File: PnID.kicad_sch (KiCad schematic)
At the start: 14 parts

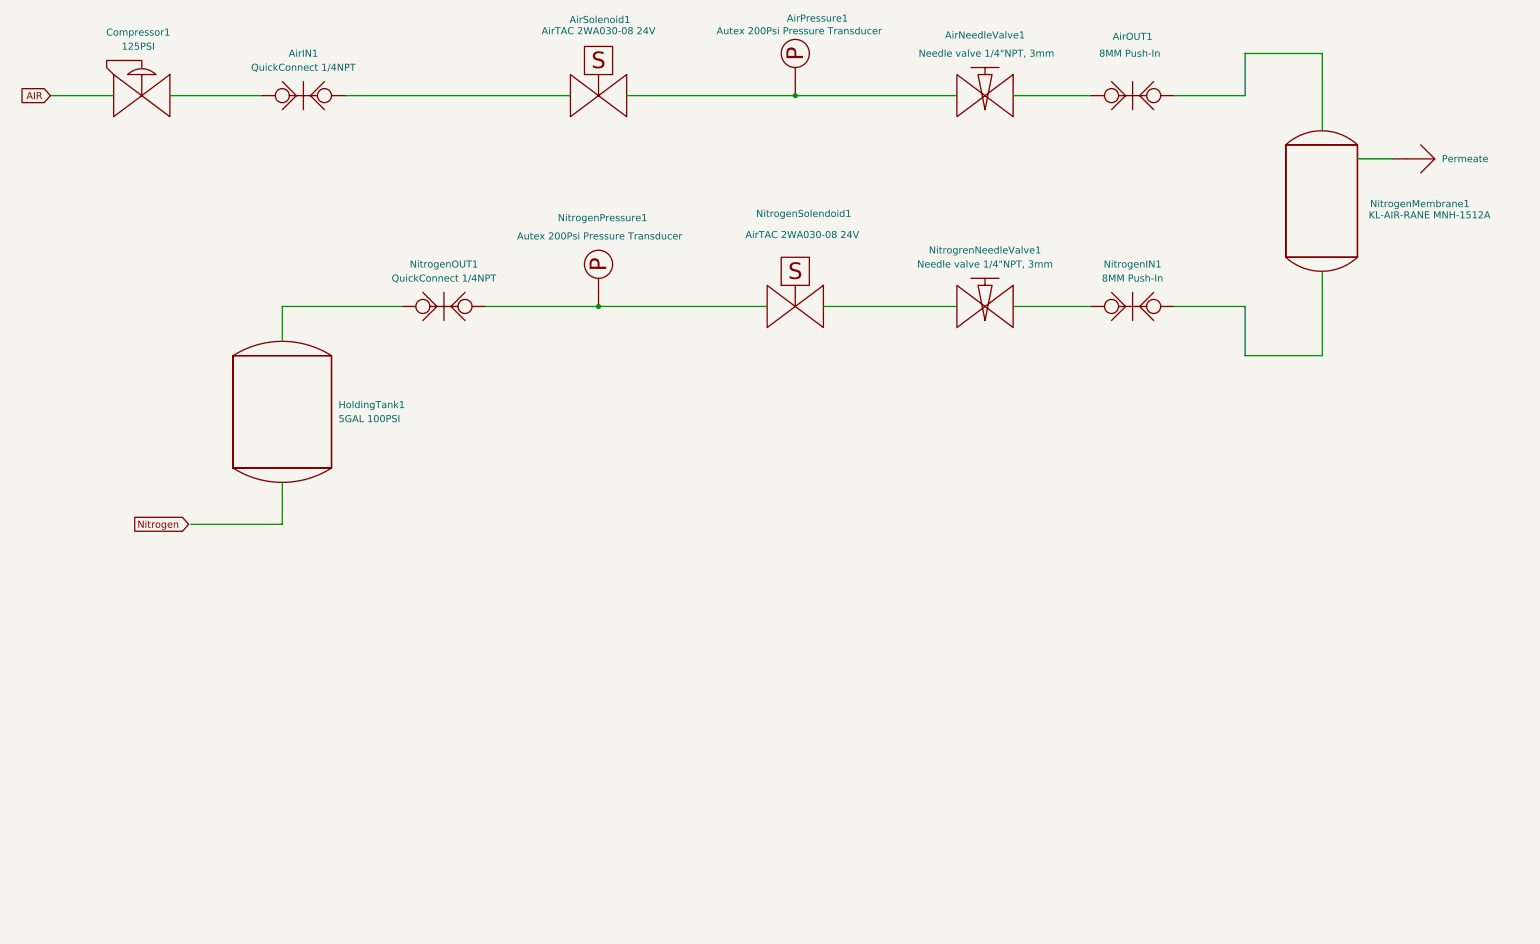
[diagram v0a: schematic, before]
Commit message: .
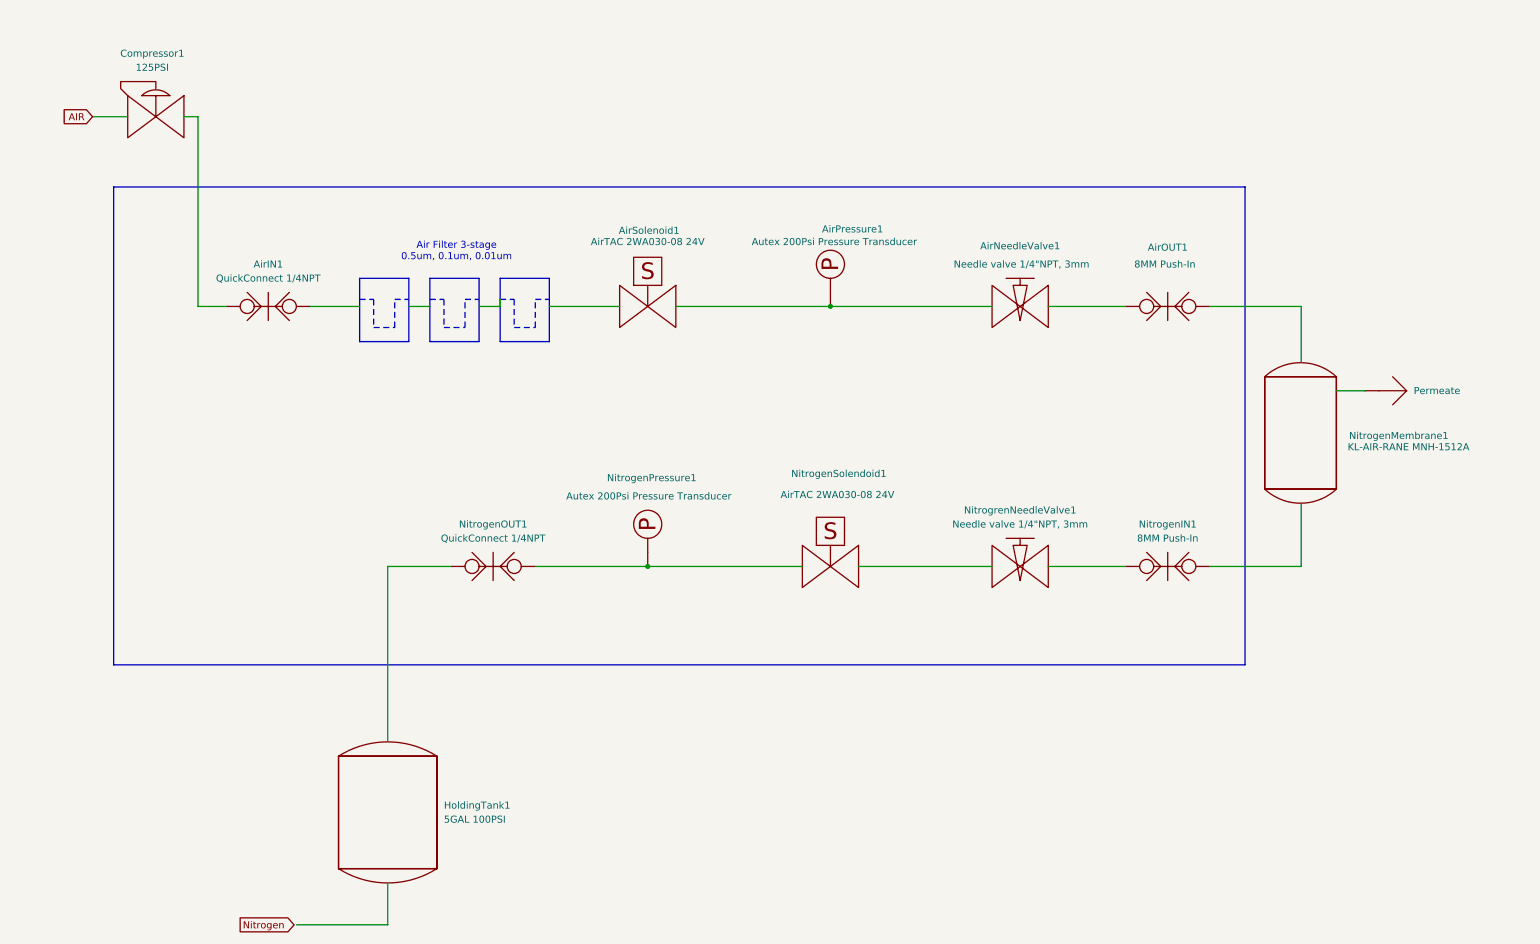
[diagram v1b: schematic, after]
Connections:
- net at NitrogenMembrane1.~: now also AirOUT1.~; no longer NitrogenIN1.~
- net at AirOUT1.~: now also AirNeedleValve1.~; no longer NitrogenMembrane1.~
- net at HoldingTank1.~: now also NitrogenOUT1.~
- net at NitrogenOUT1.~: now also NitrogenPressure1.~, NitrogenSolendoid1.~; no longer HoldingTank1.~
- net at NitrogrenNeedleValve1.~: now also NitrogenIN1.~; no longer NitrogenSolendoid1.~
- net at AirSolenoid1.~: no longer AirIN1.~
- net at AirIN1.~: no longer Compressor1.~
- new net: NitrogenIN1.~, NitrogenMembrane1.~
- new net: AirNeedleValve1.~, AirPressure1.~, AirSolenoid1.~
- new net: NitrogenSolendoid1.~, NitrogrenNeedleValve1.~
- new net: AirIN1.~, Compressor1.~
- now unconnected: AirSolenoid1.~
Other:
- note added: "Air Filter 3-stage 0.5um, 0.1um, 0.01um"
- moved on the sheet: AirIN1, AirNeedleValve1, AirOUT1, AirPressure1, AirSolenoid1, Compressor1, HoldingTank1, NitrogenIN1, NitrogenMembrane1, NitrogenOUT1, NitrogenPressure1, NitrogenSolendoid1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
